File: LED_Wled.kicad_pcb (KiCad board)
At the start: 2 copper layers, 67 x 27 mm, 22 parts, among them J1 SWD_PORT_SKEDD, J2 KF141V-2.54-2P, J3 KF141V-2.54-3P, Q1 BSS138, U1 ESP8266-12E_ESP-12E, U2 XL1509, U3 AMS1117-3.3

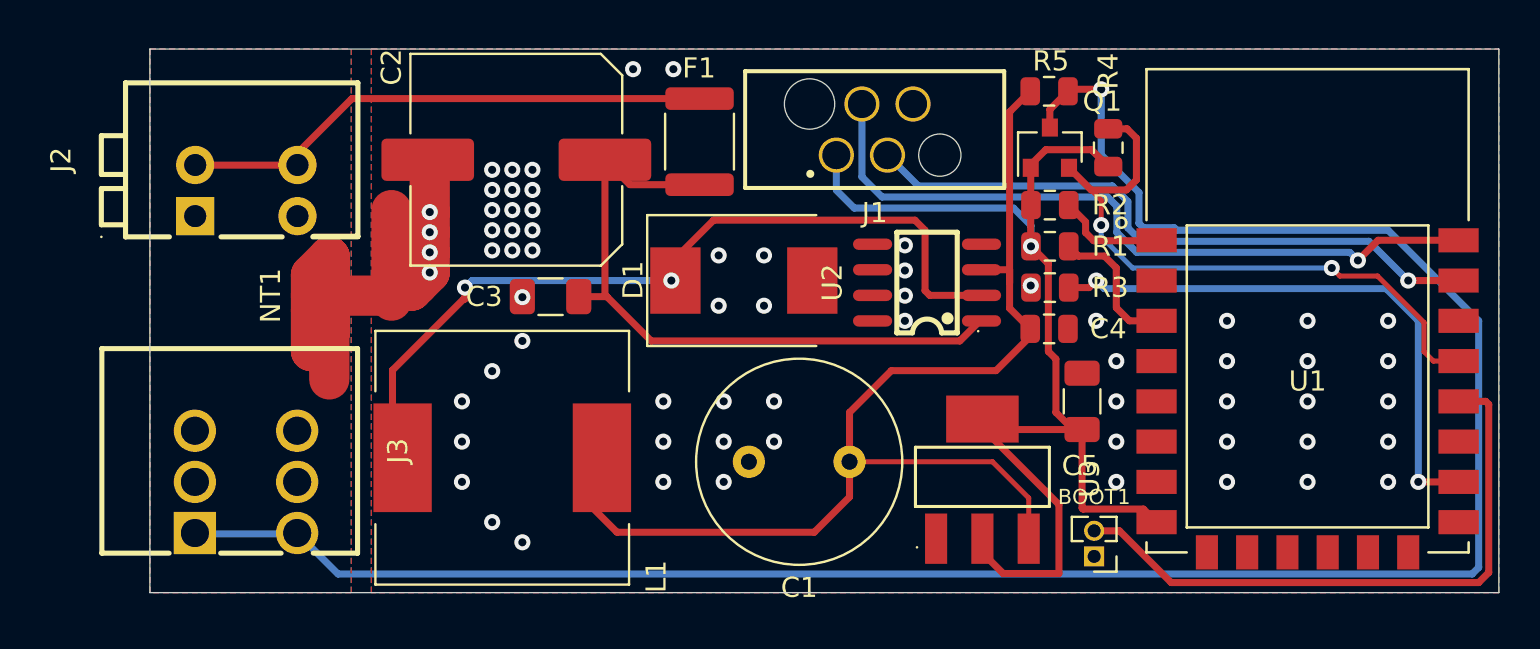
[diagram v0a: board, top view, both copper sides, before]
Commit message: new release, v1.2, prod files ready
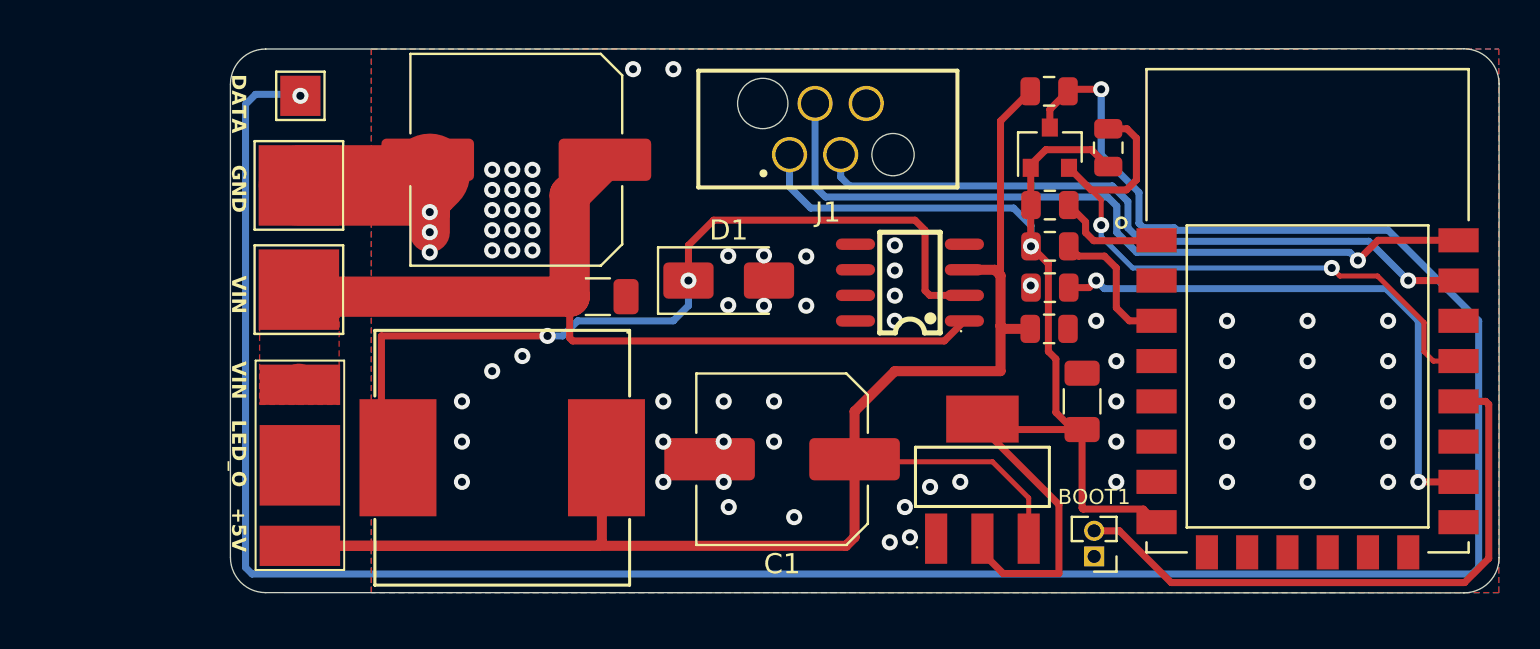
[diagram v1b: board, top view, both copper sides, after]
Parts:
- removed F1: Fuse_Small, Fuse:Fuse_1812_4532Metric
- removed NT1: Net-Tie_2, NetTie:NetTie-2_SMD_Pad2.0mm
- added J4: Conn_01x01, TestPoint:TestPoint_Pad_4.0x4.0mm, F.Cu at (73.4, 52.8)
- added JP1: SolderJumper_3_Open, LED_Wled:BIG JUMPER, F.Cu at (73.5, 65.7)
- added SYM1: LOGO, LED_Wled:easyled, B.Cu at (94.6, 59.5)
- C1: value 180uF/63V -> 220uF/35V; footprint Capacitor_THT:C_Radial_D10.0mm_H16.0mm_P5.00mm -> Capacitor_SMD:C_Elec_8x10.2
- D1: value SS32 -> SS54; footprint Diode_SMD:D_SMC -> Diode_SMD:D_SMA
- J2: value KF141V-2.54-2P -> Conn_01x01; footprint LED_Wled:CONN-TH_2P-P2.54_KF141V-2.54-2P -> TestPoint:TestPoint_Pad_4.0x4.0mm
- J3: value KF141V-2.54-3P -> Conn_01x01; footprint LED_Wled:CONN-TH_3P-P2.54_KF141V-2.54-3P -> TestPoint:TestPoint_Pad_2.0x2.0mm
- L1: footprint Inductor_SMD:L_12x12mm_H8mm -> LED_Wled:IND-SMD_L12.5-W12.5
- Q1: value BSS138 -> 2N7002
- moved J3 19.4 mm to (73.5, 48.3)
- moved J2 5.57 mm to (73.4, 58.0), turned to -90 degrees
- moved C1 3.35 mm to (97.4, 66.4)
- moved C3 2.35 mm to (88.2, 58.3), turned to 0 degrees
- moved J1 2.33 mm to (99.7, 50.0)
- moved U2 0.85 mm to (103.8, 57.6)
- moved D1 0.75 mm to (94.8, 57.5)
- turned L1 to 180 degrees
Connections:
- C2 pad 1: Net-(U2-VIN) -> VIN
- C3 pad 1: Net-(U2-VIN) -> VIN
- J2 pad 1: GNDPWR -> VIN
- U2 pad 1: Net-(U2-VIN) -> VIN
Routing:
- net Net-(U2-VIN): track 33.3 -> 0.00 mm
- net +5V: track 58.6 -> 91.3 mm
- net LED_OUT_HV: track 107.1 -> 129.9 mm, vias 1 -> 2
- net VIN: track 26.8 -> 44.1 mm
- net GNDPWR: track 16.3 -> 0.00 mm
- net RXD: track 31.7 -> 34.7 mm
- net Net-(D1-K): track 40.2 -> 42.8 mm
- net TXD: track 36.2 -> 38.8 mm
- net +3V3: track 59.4 -> 61.6 mm
- net GND: track 11.3 -> 9.74 mm, vias 66 -> 71
- added copper zone on F.Cu, net VIN
- removed copper zone on F.Cu, net GNDPWR
- removed copper zone on B.Cu, net VIN
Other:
- board size 67 x 27 mm -> 63 x 27 mm
- board text added: "DATA"
- board text added: "For use with ARGB LED-strip MAX INPUT: +24 V !SELECT INPUT BY SOLDER!"
- board text added: "GND"
- board text added: "VIN LED_O +5V"
- board text added: "wEasyLed_V1 2025-01-28 rev1.2"
- board text removed: "D_OUT"
- board text removed: "For use with ARGB LED-strip MAX INPUT: +30 V"
- board text removed: "GNDPWR"
- board text removed: "remote-led-project 2022-01-13 rev1.1"
